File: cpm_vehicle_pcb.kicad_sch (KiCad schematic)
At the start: 1 part, among them U1 4002

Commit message: schematic of battery management
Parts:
- removed U1: 4002, symbol 4xxx:4002
- added A1: BNO055, footprints_vehicle_pcb:BNO055_IMU, symbol main_board_V2.4-eagle-import:embedded_10681391_BNO055
- added C01: 10uF, footprints_vehicle_pcb:UD-4X5,8_Electrolytic_cap, symbol main_board_V2.4-eagle-import:embedded_10681391_CPOL/4X5,8
- added C02, C41, C42, C51, C53, C54, C55, C56, C61, C62: 100nF, footprints_vehicle_pcb:C0805_10681391, symbol main_board_V2.4-eagle-import:embedded_10681391_C-EUC0805
- added C31, C63, C81: 220uF, footprints_vehicle_pcb:UD-6,3X5,8_Electrolytic_CAP, symbol main_board_V2.4-eagle-import:embedded_10681391_CPOL/6,3X7,7
- added C71: 10nF, footprints_vehicle_pcb:C0805_10681391, symbol main_board_V2.4-eagle-import:embedded_10681391_C-EUC0805
- added D01: BAS40-04, footprints_vehicle_pcb:SOT23_BAS40_04_schottky_diode, symbol main_board_V2.4-eagle-import:embedded_10681391_BAS40-04
- added D2, D3: LED, LED_SMD:LED_0805_2012Metric, symbol Device:LED
- added EXT_PINS0: PINHD-2X5, footprints_vehicle_pcb:2X05_EXT_PINS, symbol main_board_V2.4-eagle-import:embedded_10681391_PINHD-2X5
- added IC1: ATMEGAAU, footprints_vehicle_pcb:TQFP100_atmega2560, symbol main_board_V2.4-eagle-import:embedded_10681391_ATMEGAAU
- added IC2: RPI-ZERO, footprints_vehicle_pcb:rpi_zero_w, symbol main_board_V2.4-eagle-import:embedded_10681391_RPI-ZERO
- added J1: Conn_02x03_Counter_Clockwise, footprints_vehicle_pcb:HARWIN_M20-9980346, symbol Connector_Generic:Conn_02x03_Counter_Clockwise
- added J2: Conn_02x03_Counter_Clockwise, footprints_vehicle_pcb:JST_B5B-XH-A, symbol Connector_Generic:Conn_02x03_Counter_Clockwise
- added J3: Conn_01x05, footprints_vehicle_pcb:PinHeader_1x05_P2.54mm_Horizontal, symbol Connector_Generic:Conn_01x05
- added J4: AVR-ISP-6, footprints_vehicle_pcb:AVR_ISP_6_footprint, symbol Connector:AVR-ISP-6
- added MCP1: ~, symbol MCP73844:MCP73844
- added P1: NCP1117, footprints_vehicle_pcb:SOT223_ncp1117, symbol main_board_V2.4-eagle-import:embedded_10681391_NCP1117
- added P2: OSTTE020104, TerminalBlock:TerminalBlock_MaiXu_MX126-5.0-02P_1x02_P5.00mm, symbol pole_screw_term_2:OSTTE020104
- added Q01: IRF3808, footprints_vehicle_pcb:TO220_IRF3808PBF, symbol main_board_V2.4-eagle-import:embedded_10681391_IRF3808
- added Q11, Q12, Q13, Q14: BSS123, footprints_vehicle_pcb:SOT23_NMOS, symbol main_board_V2.4-eagle-import:embedded_10681391_BSS123
- added QG1: XO91, footprints_vehicle_pcb:SM77H_crystal_oscillator, symbol main_board_V2.4-eagle-import:embedded_10681391_XO91
- added R/W0: PINHD-1X2/90, footprints_vehicle_pcb:1X02_90_rpi, symbol main_board_V2.4-eagle-import:embedded_10681391_PINHD-1X2/90
- added R03: 1.5k, footprints_vehicle_pcb:R0805_10681391, symbol main_board_V2.4-eagle-import:embedded_10681391_R-EUR0805
- added R04: 12k, footprints_vehicle_pcb:R0805_10681391, symbol main_board_V2.4-eagle-import:embedded_10681391_R-EUR0805
- added R05, R06: 0, footprints_vehicle_pcb:R0805_10681391, symbol main_board_V2.4-eagle-import:embedded_10681391_R-EUR0805
- added R07, R08: 560k, footprints_vehicle_pcb:R0805_10681391, symbol main_board_V2.4-eagle-import:embedded_10681391_R-EUR0805
- added R1, R2, R3o1: 1K, footprints_vehicle_pcb:R0805_10681391, symbol Device:R
- added R10, R9: 330, footprints_vehicle_pcb:R0805_10681391, symbol Device:R
- added R11, R12, R13, R14: 180, footprints_vehicle_pcb:R0805_10681391, symbol main_board_V2.4-eagle-import:embedded_10681391_R-EUR0805
- added R15, R16, R17, R18: 330, footprints_vehicle_pcb:R0805_10681391, symbol main_board_V2.4-eagle-import:embedded_10681391_R-EUR0805
- added R19: 100mΩ, PCM_JLCPCB:R_1206, symbol PCM_JLCPCB-Resistors:1206,100mΩ
- added R51: 10k 0,1%, footprints_vehicle_pcb:R0805_10681391, symbol main_board_V2.4-eagle-import:embedded_10681391_R-EUR0805
- added R52: 1k 0,1%, footprints_vehicle_pcb:R0805_10681391, symbol main_board_V2.4-eagle-import:embedded_10681391_R-EUR0805
- added Rk1, Rk2: 24k, footprints_vehicle_pcb:R0805_10681391, symbol main_board_V2.4-eagle-import:embedded_10681391_R-EUR0805
- added SI1: ~, symbol SI9433:SI9433_MOSFET
- added U1: LM385-1.2/NOPB, footprints_vehicle_pcb:SO08_LM385, symbol main_board_V2.4-eagle-import:embedded_10681391_LM385-1.2/NOPB
- added U2: LM358D, footprints_vehicle_pcb:SO08_comparator, symbol main_board_V2.4-eagle-import:embedded_10681391_LM358D
- added U3: TXB0104PWR, footprints_vehicle_pcb:TXB0104PWR, symbol main_board_V2.4-eagle-import:embedded_10681391_TXB0104PWR
- added U4: MT3608, Package_TO_SOT_SMD:SOT-23-6, symbol Regulator_Switching:MT3608
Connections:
- new net: R04.2, R05.1
- new net: R05.2, R06.1
- new net: R03.1, R04.1, U2.3 (+IN)
- new net: R03.2, Rk2.1
- new net: MCP1.7 (VBAT), SI1. (D)
- new net: MCP1.1 (SENSE), R19.2, SI1.1 (S), SI1.2 (S_1), SI1.3 (S_2)
- new net: MCP1.8 (DRV), SI1.4 (G)
- new net: D2.2 (A), R9.1
- new net: IC1.88 (PK1(ADC9/PCINT17)), R51.1, R52.2
- new net: R08.1, U1.8 (POS), U2.2 (-IN)
- new net: Rk1.1, Rk2.2
- new net: Q01.1 (G), R07.2, U2.1 (OUT)
- new net +3V3: C41.1, IC2.1 (3V3@1), U3.1 (VCCA), U3.8 (OE)
- new net +5V: A1.1 (VIN@1), C31.+, C42.1, C53.1, C54.1, C55.1, C56.1, C62.1, C63.+, C71.2, D2.1 (K), EXT_PINS0.1, IC1.10 (VCC), IC1.100 (AVCC), IC1.31 (VCC1), IC1.61 (VCC2), IC1.80 (VCC3), IC2.2 (5V0@1), IC2.4 (5V0@2), J1.1 (Pin_1), J2.1 (Pin_1), J4.2 (VCC), P1.2 (5V), P1.4 (5V), QG1.1 (E/D), QG1.4 (VCC), R1.1, R10.2, R2.1, R3o1.1, U3.14 (VCCB)
- new net /RESET: IC1.30 (RESET)
- new net AREF: C51.1, IC1.98 (AREF)
- new net BAT_GND: C01.-, C02.2, C81.-, P2.2, Q01.3 (S), R06.2, U1.4 (NG), U2.4 (V-)
- new net ERW1: EXT_PINS0.3, IC1.71 ((AD7)PA7)
- new net ERW2: EXT_PINS0.5, IC1.72 ((AD6)PA6)
- new net ERW3: EXT_PINS0.7, IC1.73 ((AD5)PA5)
- new net ERW4: EXT_PINS0.9, IC1.74 ((AD4)PA4)
- new net ERW5: EXT_PINS0.4, IC1.75 ((AD3)PA3)
- new net ERW6: EXT_PINS0.6, IC1.76 ((AD2)PA2)
- new net ERW7: EXT_PINS0.8, IC1.77 ((AD1)PA1)
- new net ERW8: EXT_PINS0.10, IC1.78 ((AD0)PA0)
- new net GND: A1.3 (GND@3), C31.-, C41.2, C42.2, C51.2, C53.2, C54.2, C55.2, C56.2, C61.2, C62.2, C63.-, C71.1, D3.1 (K), EXT_PINS0.2, IC1.11 (GND), IC1.32 (GND1), IC1.62 (GND2), IC1.81 (GND3), IC1.99 (AGND), IC2.14 (GND@4), IC2.20 (GND@5), IC2.25 (GND@2), IC2.30 (GND@6), IC2.34 (GND@7), IC2.39 (GND@3), IC2.6 (GND@8), IC2.9 (GND@1), J1.6 (Pin_6), J2.6 (Pin_6), J3.3 (Pin_3), J3.4 (Pin_4), J4.6 (GND), P1.1 (GND), Q01.2 (D), Q11.2 (S), Q12.2 (S), Q13.2 (S), Q14.2 (S), QG1.2 (GND), R/W0.1, R52.1, R9.2, U3.7 (GND)
- new net LED1: IC1.26 ((OC0A/OC1C/PCINT7)PB7), R11.1
- new net LED1_PIN: J1.3 (Pin_3), R15.2
- new net LED2: IC1.27 (PH7(T4)), R12.1
- new net LED2_PIN: J1.4 (Pin_4), R16.2
- new net LED3: IC1.18 (PH6(OC2B)), R13.1
- new net LED3_PIN: J1.2 (Pin_2), R17.2
- new net LED4: IC1.17 (PH5(OC4C)), R14.1
- new net LED4_PIN: J1.5 (Pin_5), R18.2
- new net LED_BUILT_IN: D3.2 (A), IC1.54 ((A9)PC1), R10.1
- new net MISO: IC1.22 ((MISO/PCINT3)PB3), J4.1 (MISO), U3.10 (B4)
- new net MISO_PI: IC2.21 (GPIO9/MISO), U3.5 (A4)
- new net MODE: IC2.29 (GPIO5), R/W0.2
- new net MOSI: IC1.21 ((MOSI/PCINT2)PB2), J4.4 (MOSI), U3.11 (B3)
- new net MOSI_PI: IC2.19 (GPIO10/MOSI), U3.4 (A3)
- new net PWM: IC1.8 ((T3/INT6)PE6), J3.5 (Pin_5)
- new net R11: Q11.1 (G), R11.2
- new net R12: Q12.1 (G), R12.2
- new net R13: Q13.1 (G), R13.2
- new net R14: Q14.1 (G), R14.2
- new net R15: Q11.3 (D), R15.1
- new net R16: Q12.3 (D), R16.1
- new net R17: Q13.3 (D), R17.1
- new net R18: Q14.3 (D), R18.1
- new net SCK: IC1.20 ((SCK/PCINT1)PB1), J4.3 (SCK), U3.12 (B2)
- new net SCK_PI: IC2.23 (GPIO11/SCLK), U3.3 (A2)
- new net SCL: A1.5 (SCL@5), IC1.43 ((SCL/INT0)PD0)
- new net SDA: A1.4 (SDA@4), IC1.44 ((SDA/INT1)PD1)
- new net SENSOR1: IC1.85 (PK4(ADC12/PCINT20)), J2.3 (Pin_3), R1.2
- new net SENSOR2: IC1.86 (PK3(ADC11/PCINT19)), J2.5 (Pin_5), R2.2
- new net SENSOR3: IC1.87 (PK2(ADC10/PCINT18)), J2.2 (Pin_2), R3o1.2
- new net SERVO_PWM: J3.1 (Pin_1)
- new net SS: IC1.19 ((SS/PCINT0)PB0), U3.13 (B1)
- new net SS_PI: IC2.24 (~{CE0}/GPIO8), U3.2 (A1)
- new net TCK: IC1.93 ((ADC4/TCK)PF4)
- new net TDI: IC1.90 ((ADC7/TDI)PF7)
- new net TDO: IC1.91 ((ADC6/TDO)PF6)
- new net TMS: IC1.92 ((ADC5/TMS)PF5)
- new net VCC_BAT: C61.1, C81.+, D01.1 (A1), J3.2 (Pin_2), P1.3 (VIN), P2.1, R51.2
- new net VCC_BAT_LP: C01.+, C02.1, D01.3 (C1A2), R08.2, Rk1.2, U2.8 (V+)
- new net XTAL1: IC1.34 (XTAL1), QG1.3 (OUT)
- new net /RESET: J4.5 (~{RST})
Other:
- note added: "(For Powering ESC)"
- note added: "A side Vcc from 1.2 to 3.6V"
- note added: "B side Vcc from 1.65 to 5V"
- note added: "Battery monitoring system"
- note added: "VccA *must* be less than VccB~{}"

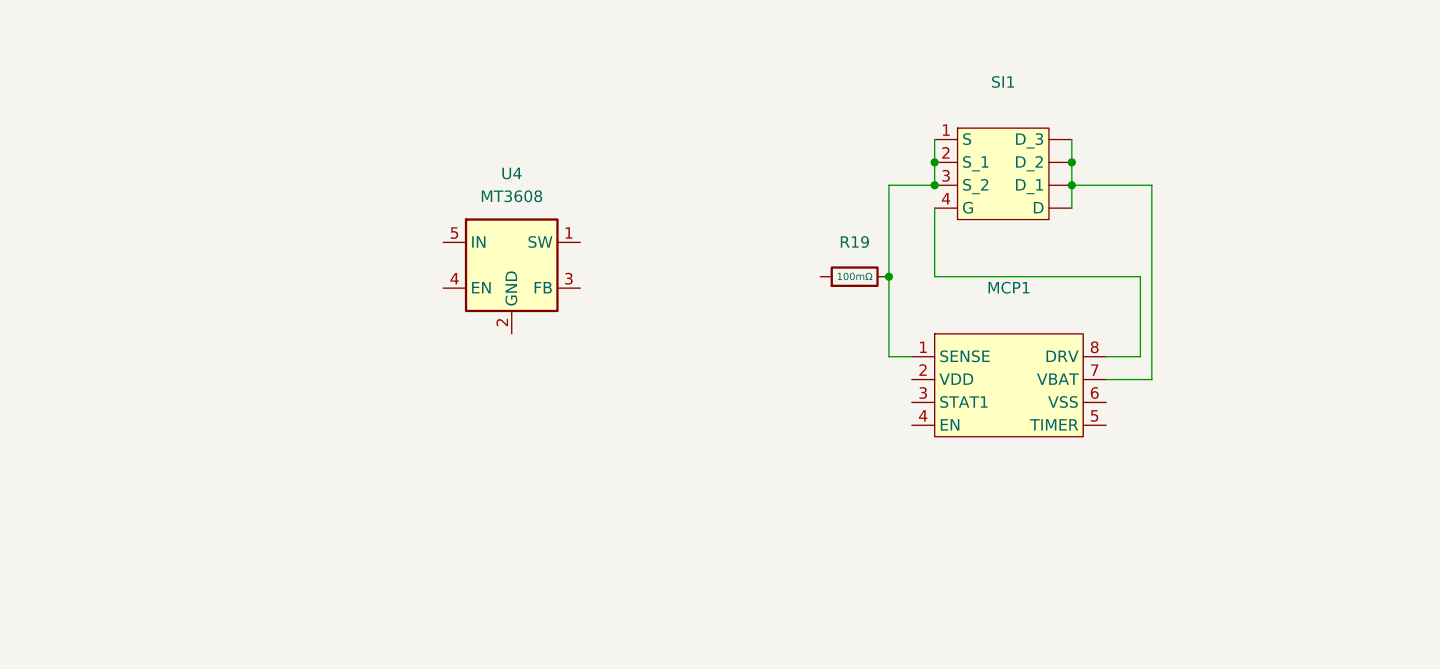
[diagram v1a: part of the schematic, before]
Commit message: update
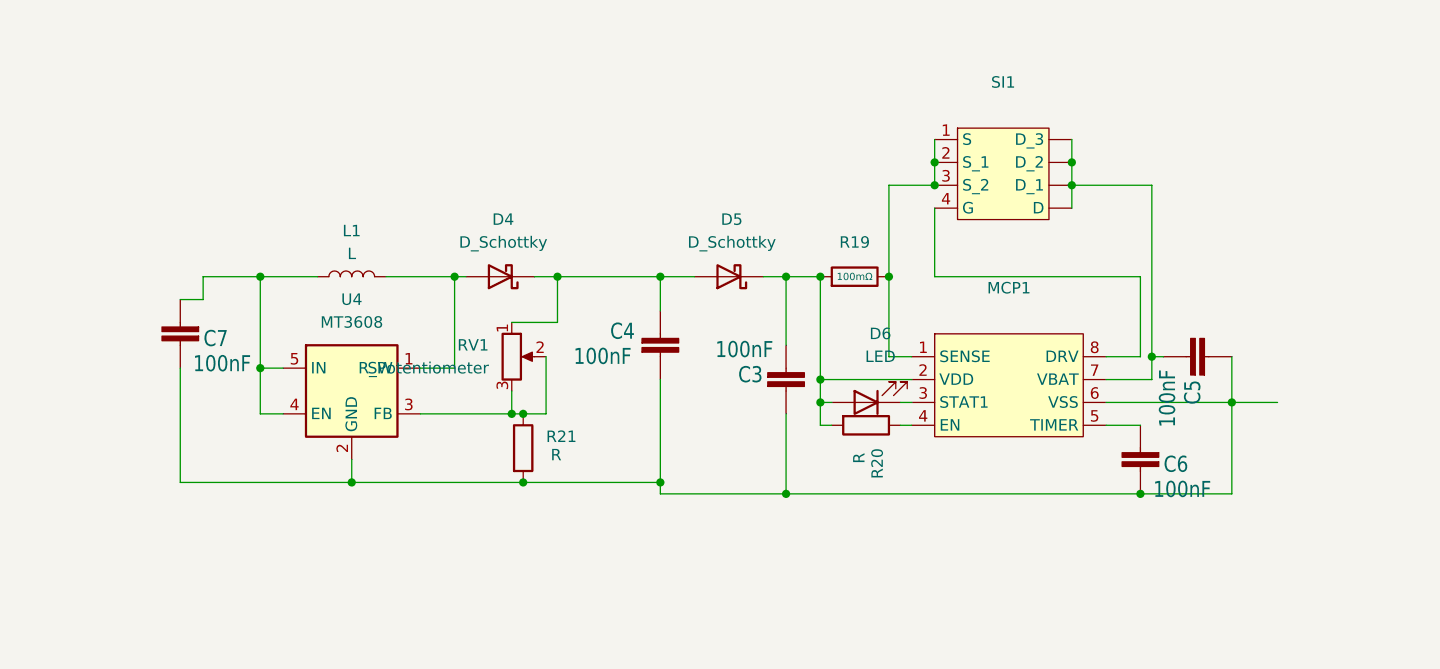
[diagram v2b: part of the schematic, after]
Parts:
- added C3, C4, C5, C6, C7: 100nF, footprints_vehicle_pcb:C0805_10681391, symbol main_board_V2.4-eagle-import:embedded_10681391_C-EUC0805
- added D4, D5: D_Schottky, symbol Device:D_Schottky
- added D6: LED, symbol Device:LED
- added L1: L, symbol Device:L
- added R20, R21: R, symbol Device:R
- added RV1: R_Potentiometer, symbol Device:R_Potentiometer
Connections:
- net at U4.1 (SW): now also D4.2 (A), L1.2
- net at U4.2 (GND): now also MCP1.6 (VSS), C3.2, C4.2, C5.2, C6.1, C7.1, R21.2
- net at U4.3 (FB): now also R21.1, RV1.2, RV1.3
- net at U4.4 (EN): now also U4.5 (IN), C7.2, L1.1
- net at MCP1.7 (VBAT), SI1. (D): now also C5.1
- net at R19.1: now also MCP1.2 (VDD), C3.1, D5.1 (K), D6.2 (A), R20.2
- net at MCP1.3 (STAT1): now also D6.1 (K)
- net at MCP1.4 (EN): now also R20.1
- net at MCP1.5 (TIMER): now also C6.2
- new net: C4.1, D4.1 (K), D5.2 (A), RV1.1
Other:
- moved on the sheet: U4
